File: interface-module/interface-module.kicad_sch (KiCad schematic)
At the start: 54 parts, among them J2 Conn_01x02, J4 Conn_01x08, J6 Conn_01x08, SW1 SW_Coded_SH-7050, U10 TCA9548, U11 MCP3464

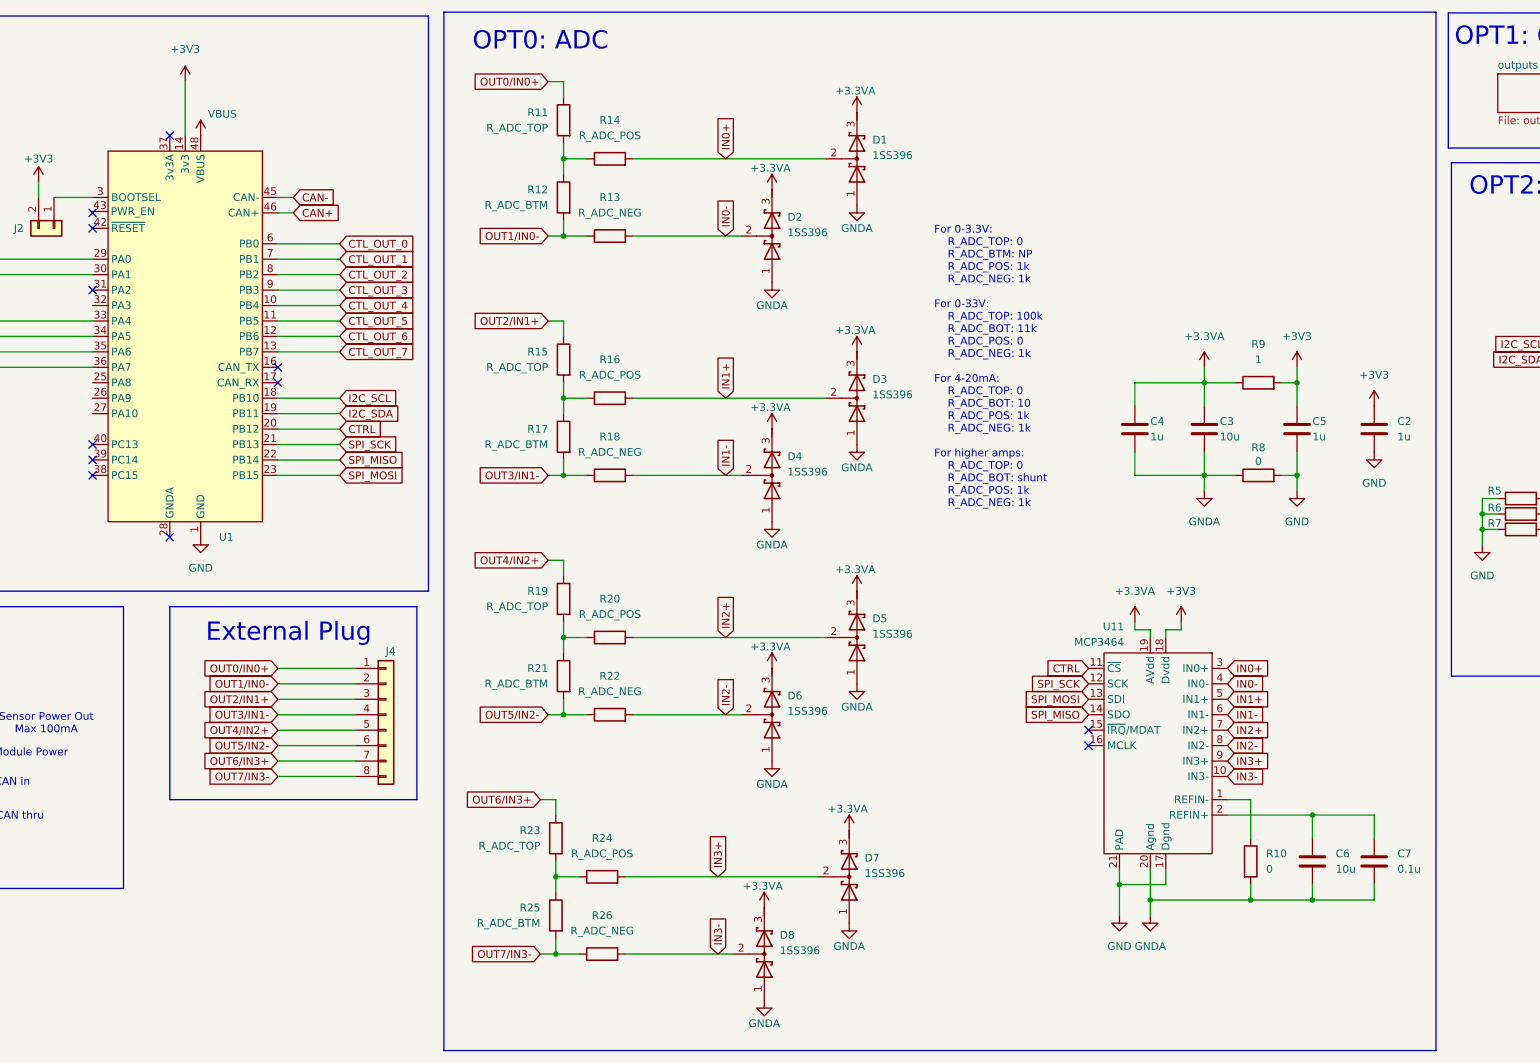
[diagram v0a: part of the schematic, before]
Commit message: Finished copper layout
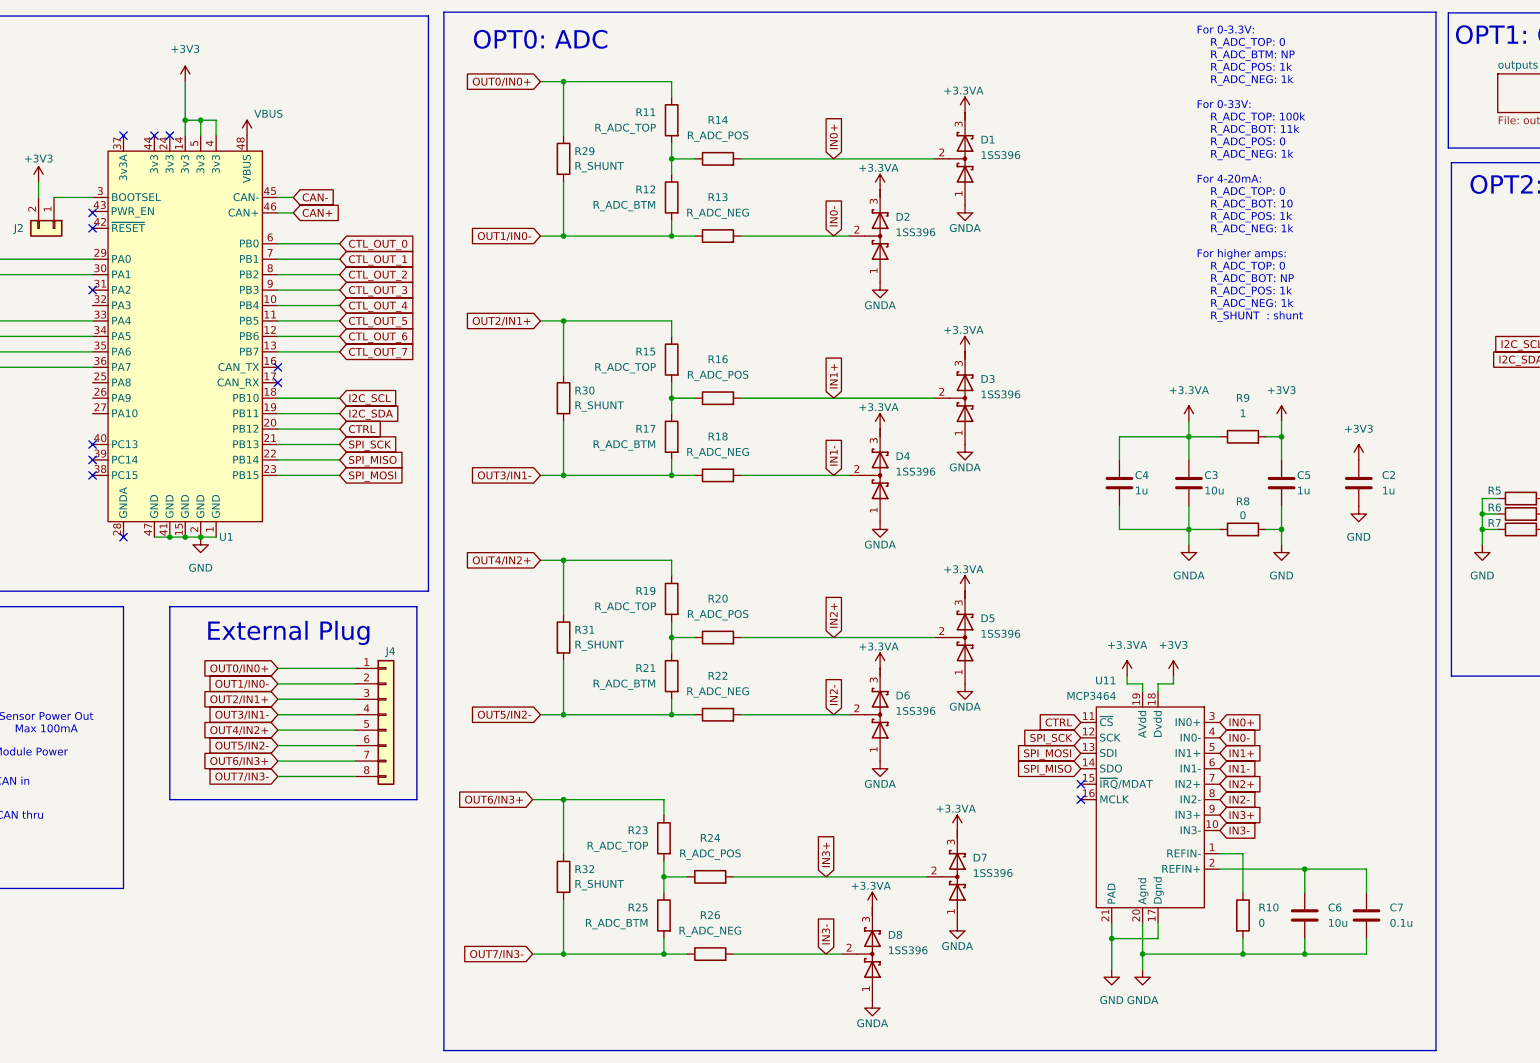
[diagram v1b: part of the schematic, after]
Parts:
- added R29, R30, R31, R32: R_SHUNT, Resistor_SMD:R_0603_1608Metric, symbol Device:R
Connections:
- net +3V3: no longer U1.24 (3v3), U1.44 (3v3)
- net OUT0/IN0+: now also R29.1
- net OUT1/IN0-: now also R29.2
- net OUT2/IN1+: now also R30.1
- net OUT3/IN1-: now also R30.2
- net OUT4/IN2+: now also R31.1
- net OUT5/IN2-: now also R31.2
- net OUT6/IN3+: now also R32.1
- net OUT7/IN3-: now also R32.2
- no-connect marks 20 -> 22
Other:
- note added: "For 0-3.3V: R_ADC_TOP: 0 R_ADC_BTM: NP R_ADC_POS: 1k R_ADC_NEG: 1k For 0-33V: R_ADC_TOP: 100k R_ADC_BOT: 11k R_ADC_POS: 0 R_ADC_NEG: 1k For 4-20mA: R_ADC_TOP: 0 R_ADC_BOT: 10 R_ADC_POS: 1k R_ADC_NEG: 1k For higher amps: R_ADC_TOP: 0 R_ADC_BOT: NP R_ADC_POS: 1k R_ADC_NEG: 1k R_SHUNT : shunt"
- note removed: "For 0-3.3V: R_ADC_TOP: 0 R_ADC_BTM: NP R_ADC_POS: 1k R_ADC_NEG: 1k For 0-33V: R_ADC_TOP: 100k R_ADC_BOT: 11k R_ADC_POS: 0 R_ADC_NEG: 1k For 4-20mA: R_ADC_TOP: 0 R_ADC_BOT: 10 R_ADC_POS: 1k R_ADC_NEG: 1k For higher amps: R_ADC_TOP: 0 R_ADC_BOT: shunt R_ADC_POS: 1k R_ADC_NEG: 1k"
- moved on the sheet: C2, C3, C4, C5, C6, C7, D1, D2, D3, D4, D5, D6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
